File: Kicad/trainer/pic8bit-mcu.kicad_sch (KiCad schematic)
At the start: 23 parts, among them K201 MCU 1, K202 MCU 2, K203 ICSP, K204 VIN, K205 VIN, K206 VDD, K207 GND, K208 VDD, K209 GND, K210 HARWIN-254-F-1X10-VERTICAL, U201 PIC16F/18F, X1 XTAL-DIL08

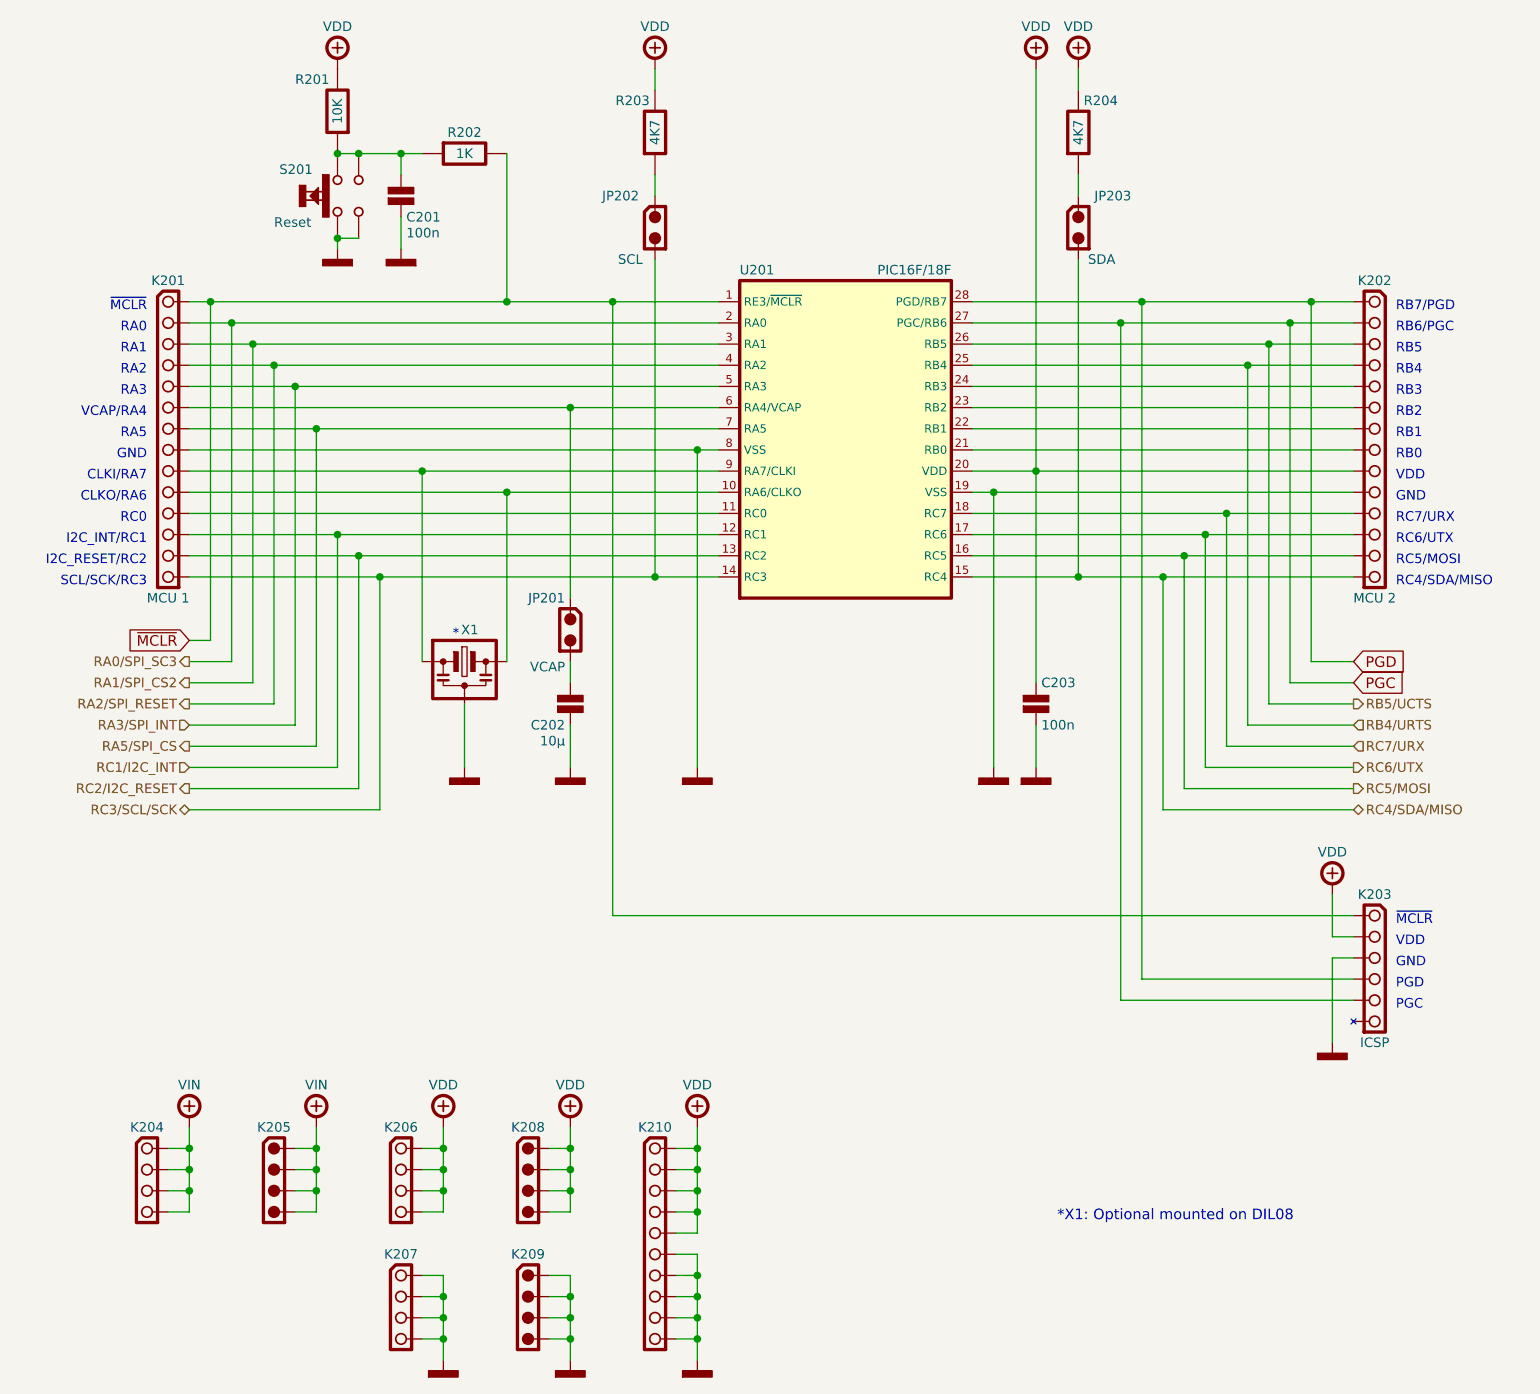
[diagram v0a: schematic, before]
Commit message: Update
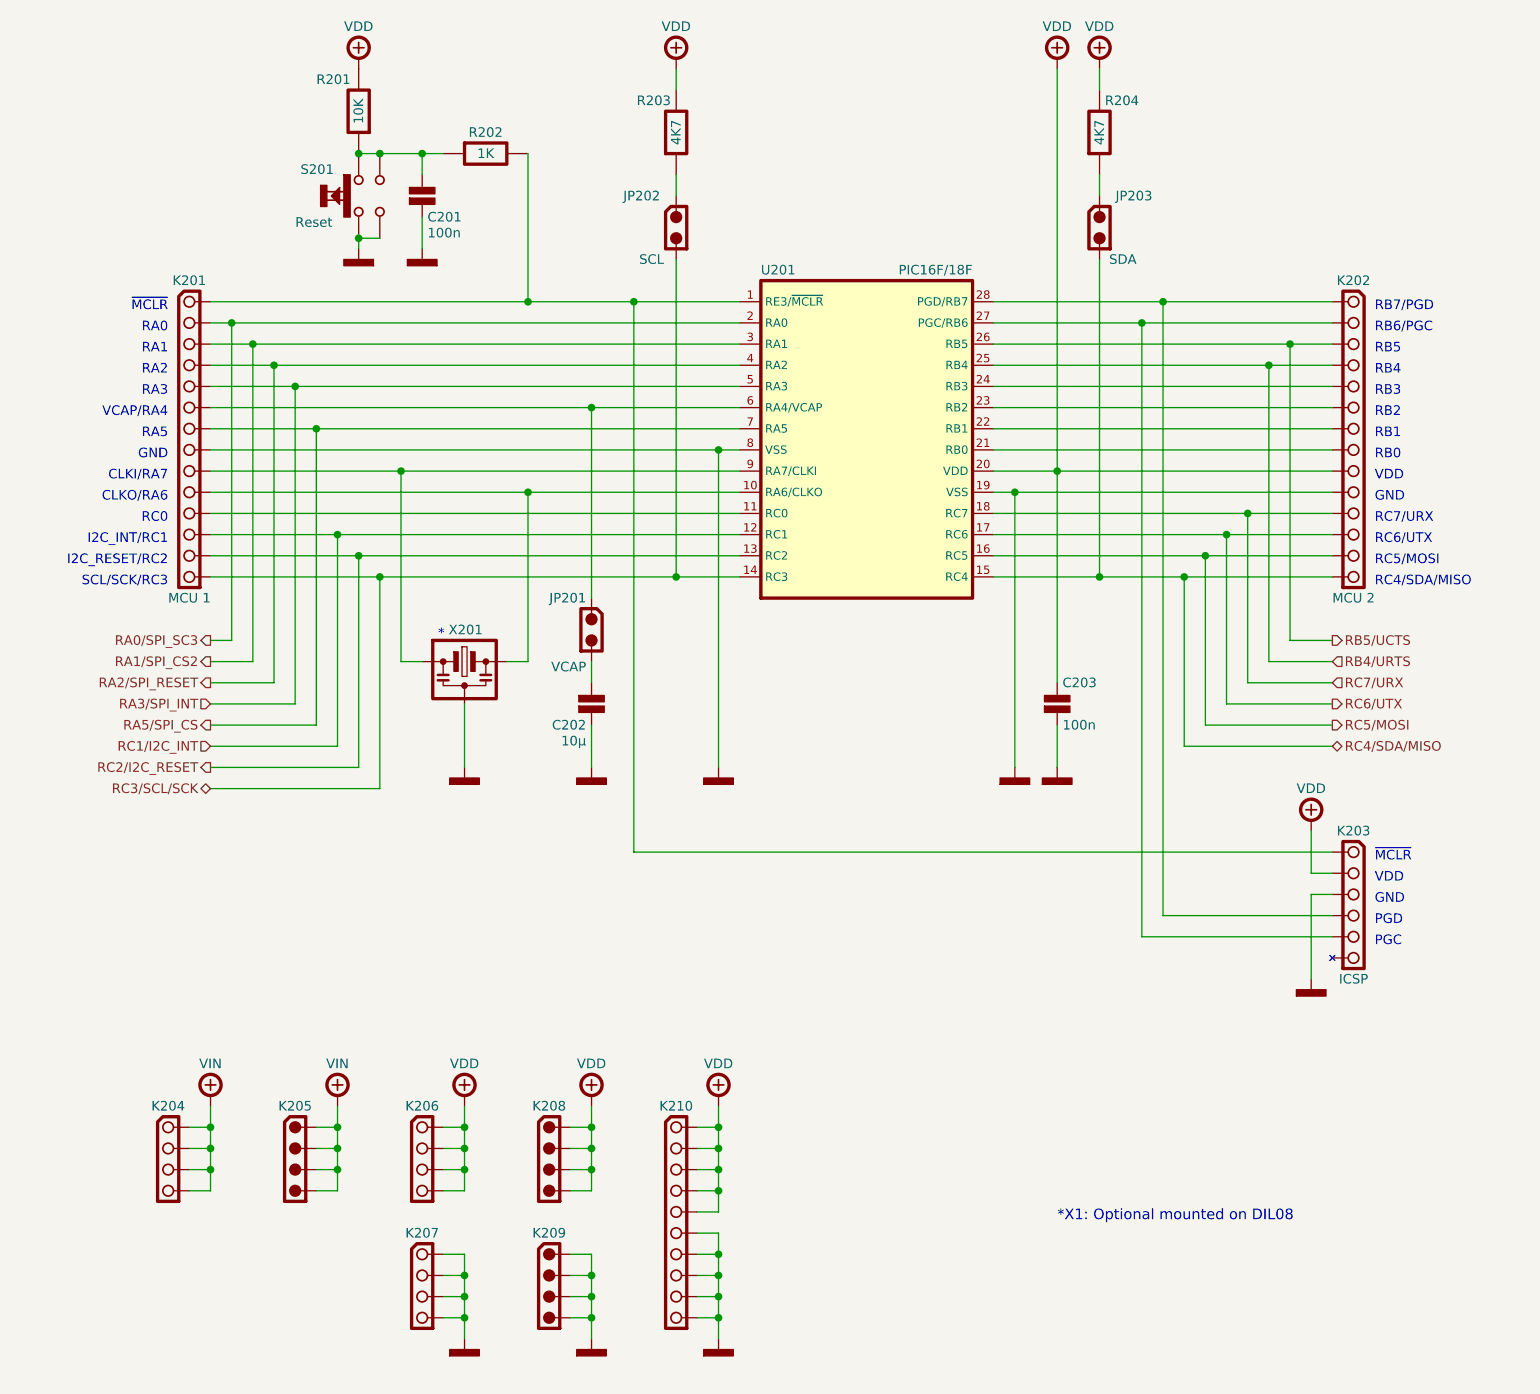
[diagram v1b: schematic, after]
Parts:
- renumbered X1 to X201
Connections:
- net PGC: no longer names the net of K202.2 (Pin_2), K203.2, U201.27 (PGC/RB6)
- net PGD: no longer names the net of K202.1 (Pin_1), K203.3, U201.28 (PGD/RB7)
- net ~{MCLR}: no longer names the net of K201.1 (Pin_1), K203.6, R202.1, U201.1 (RE3/~{MCLR})
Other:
- moved on the sheet: C201, C202, C203, JP201, JP202, JP203, K201, K202, K203, K204, K205, K206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
